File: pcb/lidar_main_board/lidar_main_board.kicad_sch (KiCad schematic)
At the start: 18 parts, among them J1 vl53l1x, J2 AS5600, J3 HC-06, J4 Bateria, U1 LPC845-BRK, U2 AMS1117-3.3, U3 LM7805_TO220

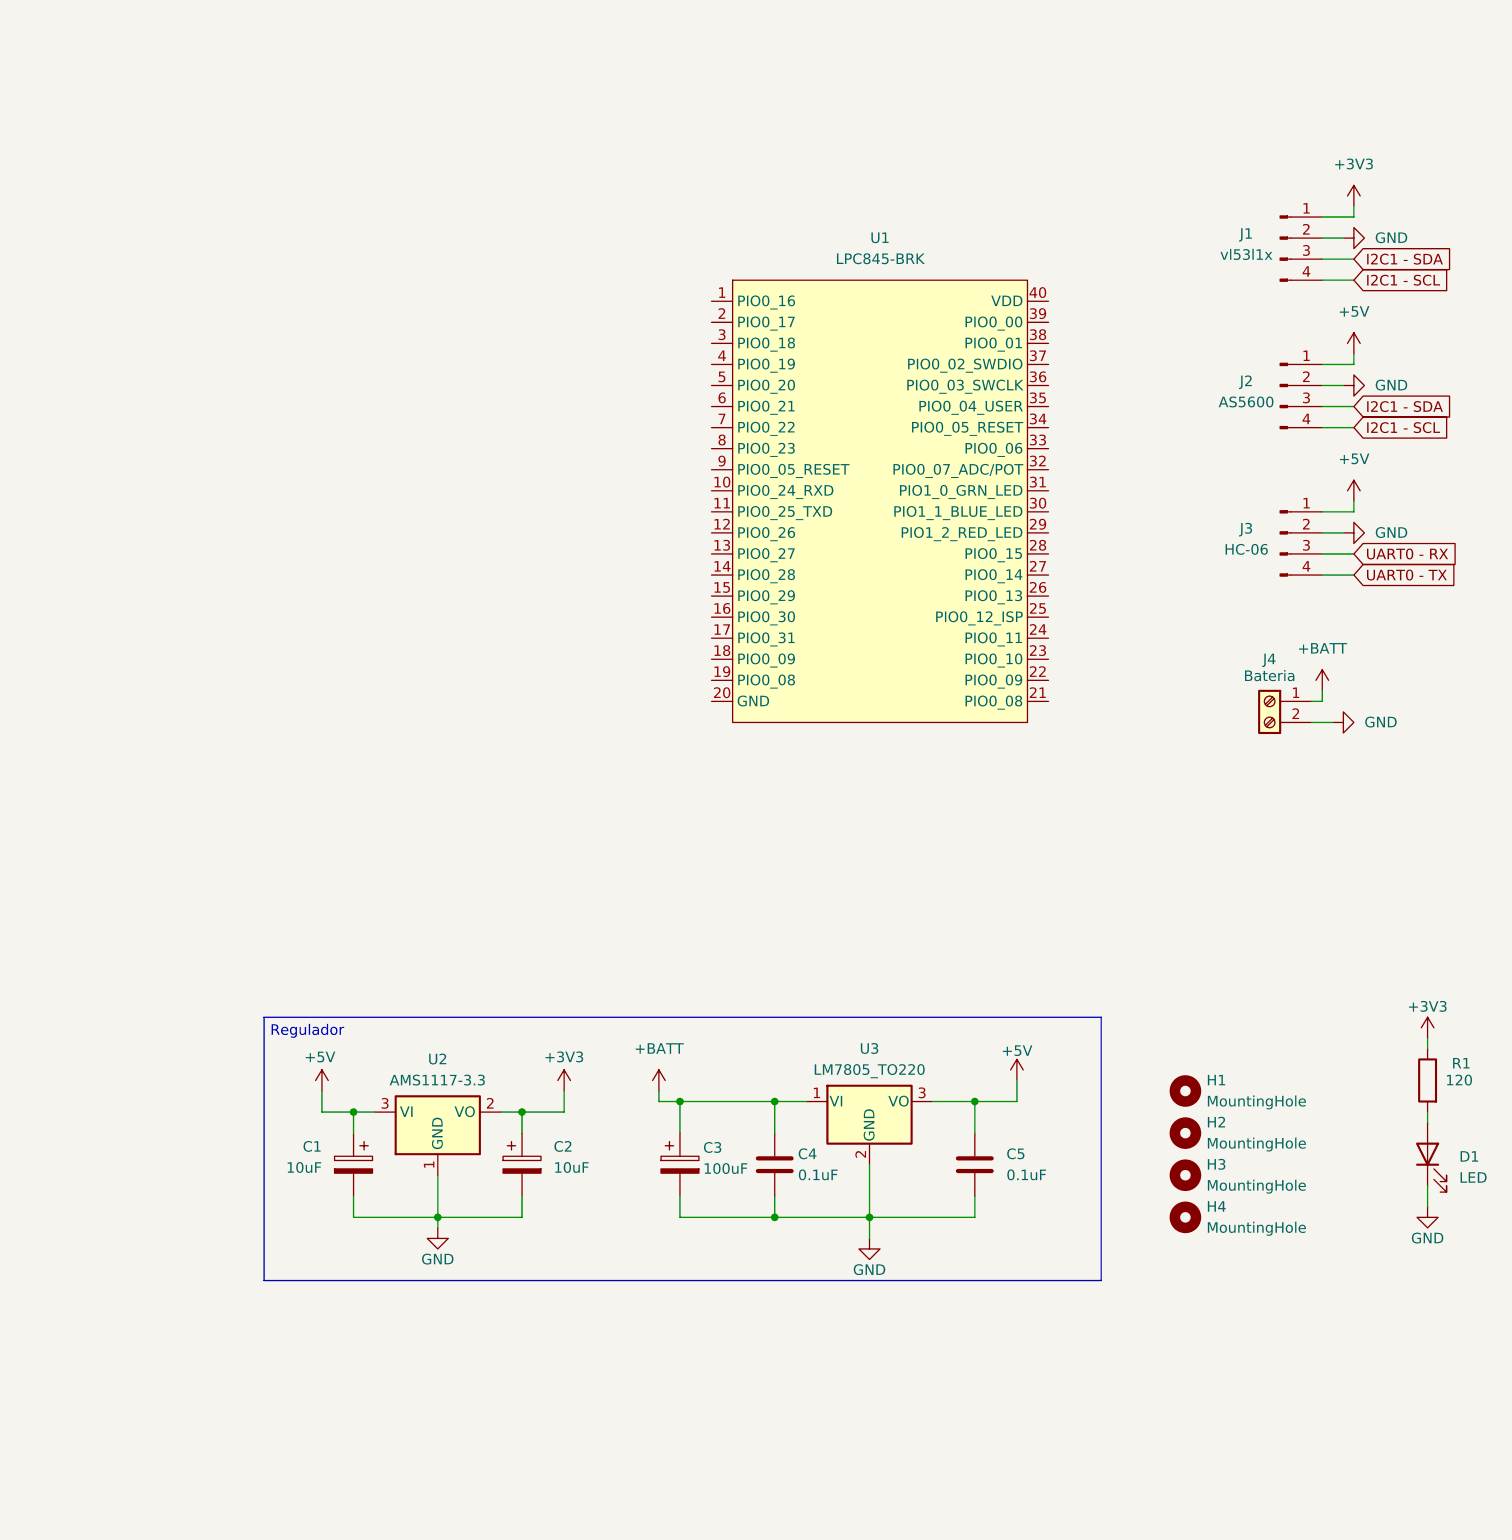
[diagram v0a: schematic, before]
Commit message: add pcb
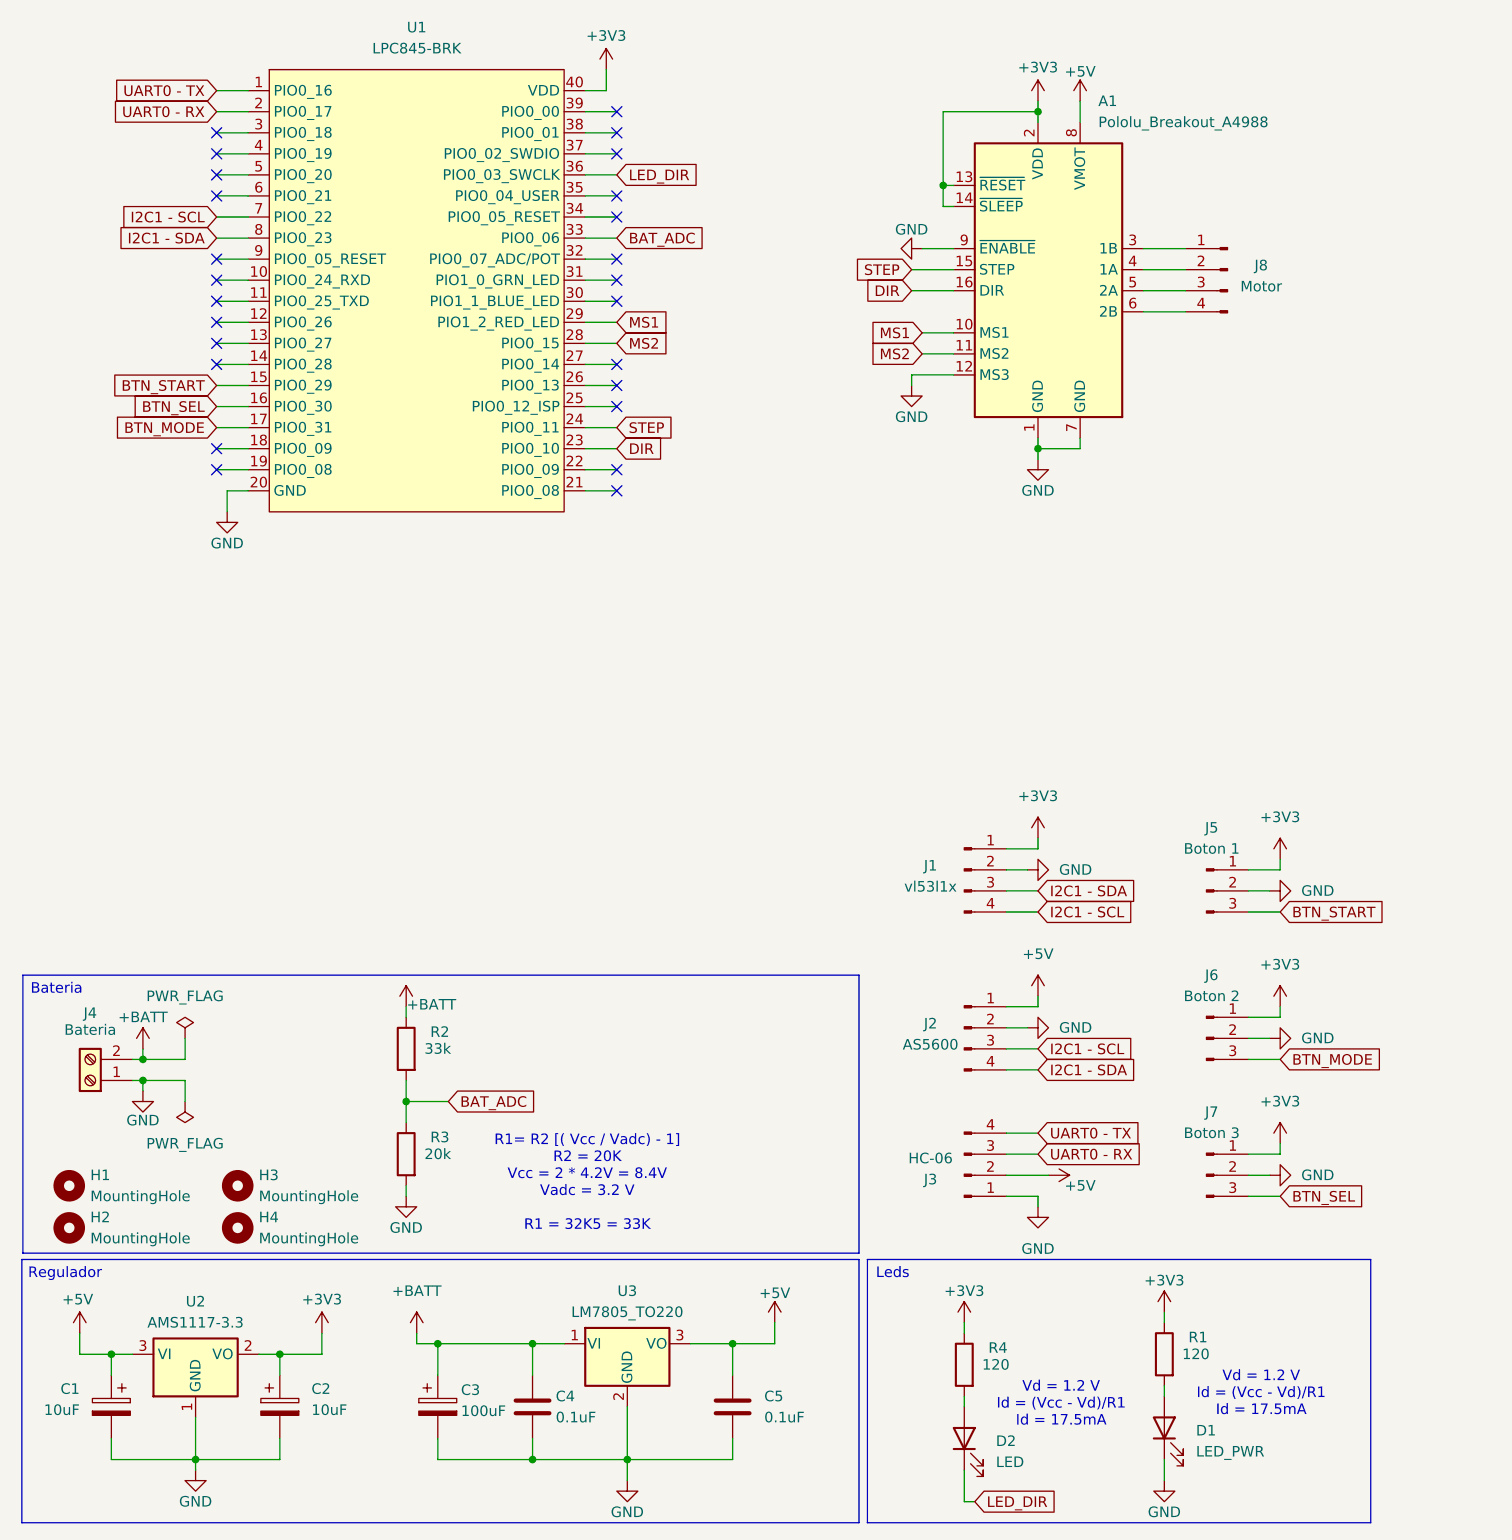
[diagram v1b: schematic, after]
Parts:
- added A1: Pololu_Breakout_A4988, Module:Pololu_Breakout-16_15.2x20.3mm, symbol Driver_Motor:Pololu_Breakout_A4988
- added D2: LED, LED_THT:LED_D5.0mm, symbol Device:LED
- added J5: Boton 1, Connector_PinHeader_2.54mm:PinHeader_1x03_P2.54mm_Vertical, symbol Connector:Conn_01x03_Pin
- added J6: Boton 2, Connector_PinHeader_2.54mm:PinHeader_1x03_P2.54mm_Vertical, symbol Connector:Conn_01x03_Pin
- added J7: Boton 3, Connector_PinHeader_2.54mm:PinHeader_1x03_P2.54mm_Vertical, symbol Connector:Conn_01x03_Pin
- added J8: Motor, Connector_PinHeader_2.54mm:PinHeader_1x04_P2.54mm_Vertical, symbol Connector:Conn_01x04_Pin
- added R2: 33k, Resistor_THT:R_Axial_DIN0207_L6.3mm_D2.5mm_P10.16mm_Horizontal, symbol Device:R
- added R3: 20k, Resistor_THT:R_Axial_DIN0207_L6.3mm_D2.5mm_P10.16mm_Horizontal, symbol Device:R
- added R4: 120, Resistor_THT:R_Axial_DIN0207_L6.3mm_D2.5mm_P10.16mm_Horizontal, symbol Device:R
- D1: value LED -> LED_PWR
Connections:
- net +3V3: now also U1.40 (VDD), A1.13 (~{RESET}), A1.14 (~{SLEEP}), A1.2 (VDD), J5.1 (Pin_1), J6.1 (Pin_1), J7.1 (Pin_1), R4.1
- net +5V: now also J3.2 (Pin_2), A1.8 (VMOT); no longer J3.1 (Pin_1)
- net +BATT: now also J4.2 (Pin_2), R2.1; no longer J4.1 (Pin_1)
- net GND: now also J3.1 (Pin_1), J4.1 (Pin_1), U1.20 (GND), A1.1 (GND), A1.12 (MS3), A1.7 (GND), A1.9 (~{ENABLE}), J5.2 (Pin_2), J6.2 (Pin_2), J7.2 (Pin_2), R3.2; no longer J3.2 (Pin_2), J4.2 (Pin_2)
- net I2C1 - SCL: now also J2.3 (Pin_3), U1.7 (PIO0_22); no longer J2.4 (Pin_4)
- net I2C1 - SDA: now also J2.4 (Pin_4), U1.8 (PIO0_23); no longer J2.3 (Pin_3)
- net UART0 - RX: now also U1.2 (PIO0_17)
- net UART0 - TX: now also U1.1 (PIO0_16)
- net BTN_START: now reaches U1.15 (PIO0_29)
- net BTN_START: now also J5.3 (Pin_3)
- net BTN_SEL: now reaches U1.16 (PIO0_30)
- net BTN_SEL: now also J7.3 (Pin_3)
- net BTN_MODE: now reaches U1.17 (PIO0_31)
- net BTN_MODE: now also J6.3 (Pin_3)
- net DIR: now reaches U1.23 (PIO0_10)
- net DIR: now also A1.16 (DIR)
- net STEP: now reaches U1.24 (PIO0_11)
- net STEP: now also A1.15 (STEP)
- net MS2: now reaches U1.28 (PIO0_15)
- net MS2: now also A1.11 (MS2)
- net MS1: now reaches U1.29 (PIO1_2_RED_LED)
- net MS1: now also A1.10 (MS1)
- net BAT_ADC: now reaches U1.33 (PIO0_06)
- net BAT_ADC: now also R2.2, R3.1
- net LED_DIR: now reaches U1.36 (PIO0_03_SWCLK)
- net LED_DIR: now also D2.1 (K)
- new net: D2.2 (A), R4.2
- new net: A1.3 (1B), J8.1 (Pin_1)
- new net: A1.4 (1A), J8.2 (Pin_2)
- new net: A1.5 (2A), J8.3 (Pin_3)
- new net: A1.6 (2B), J8.4 (Pin_4)
- no-connect marks 0 -> 25
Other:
- note added: "Bateria"
- note added: "Leds"
- note added: "R1= R2 [( Vcc / Vadc) - 1] R2 = 20K Vcc = 2 * 4.2V = 8.4V Vadc = 3.2 V R1 = 32K5 = 33K"
- note added: "Vd = 1.2 V Id = (Vcc - Vd)/R1 Id = 17.5mA"
- moved on the sheet: C1, C2, C3, C4, C5, D1, H1, H2, H3, H4, J1, J2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
